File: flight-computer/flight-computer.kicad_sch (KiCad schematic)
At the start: 37 parts, among them J1 Conn_01x06_Pin, J2 Conn_01x06_Pin, J3 Power Connector, J4 Micro_SD_Card, J5 USB_C_Receptacle_USB2.0_16P, J6 Conn_01x02_Pin, Q1 DMN3404L, Q2 DMN3404L, U1 LMR51420X, U2 ESP32-S3-WROOM-1, U3 LSM6DSO32TR, U4 INA2180A1IDGKR

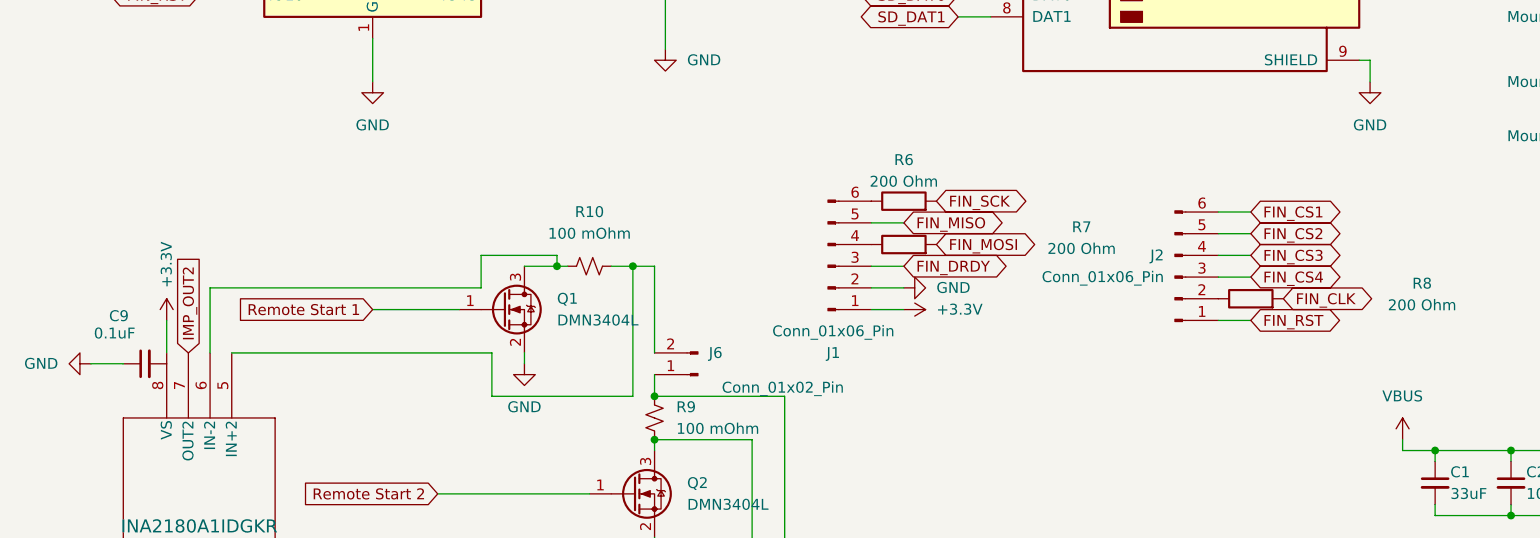
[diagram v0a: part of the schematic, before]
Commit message: finished connecting things
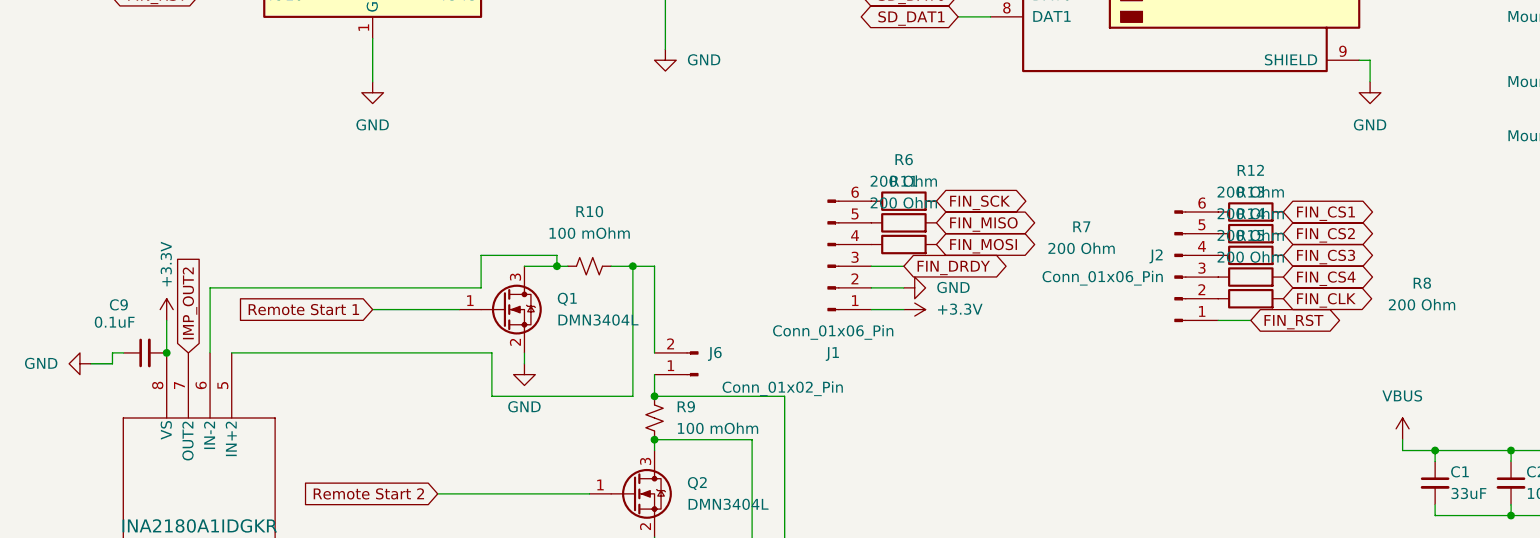
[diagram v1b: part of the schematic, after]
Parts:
- added R11, R12, R13, R14, R15: 200 Ohm, Resistor_SMD:R_0402_1005Metric, symbol Device:R
- J1, J2: footprint Connector_JST:JST_ZH_S6B-ZR-SM4A-TF_1x06-1MP_P1.50mm_Horizontal -> Connector_JST:JST_ZE_S06B-ZESK-2D_1x06_P1.50mm_Horizontal
- R10, R9: footprint Resistor_SMD:R_0402_1005Metric -> Resistor_SMD:R_1206_3216Metric
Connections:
- net +3.3V: now also C9.2
- net FIN_CS1: now also R12.2; no longer J2.6 (Pin_6)
- net FIN_CS2: now also R13.2; no longer J2.5 (Pin_5)
- net FIN_CS3: now also R14.2; no longer J2.4 (Pin_4)
- net FIN_CS4: now also R15.2; no longer J2.3 (Pin_3)
- net FIN_MISO: now also R11.2; no longer J1.5 (Pin_5)
- new net: J1.5 (Pin_5), R11.1
- new net: J2.3 (Pin_3), R15.1
- new net: J2.4 (Pin_4), R14.1
- new net: J2.5 (Pin_5), R13.1
- new net: J2.6 (Pin_6), R12.1
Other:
- moved on the sheet: C9

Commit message: started organizing
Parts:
- J1, J2: footprint Connector_JST:JST_ZE_S06B-ZESK-2D_1x06_P1.50mm_Horizontal -> Connector_JST:JST_ZE_SM06B-ZESS-TB_1x06-1MP_P1.50mm_Horizontal
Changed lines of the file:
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@@
 			)
 		)
-		(property "Footprint" "Connector_JST:JST_ZE_S06B-ZESK-2D_1x06_P1.50mm_Horizontal"
+		(property "Footprint" "Connector_JST:JST_ZE_SM06B-ZESS-TB_1x06-1MP_P1.50mm_Horizontal"
 			(at 163.83 116.84 0)
 			(effects
@@
 			)
 		)
-		(property "Footprint" "Connector_JST:JST_ZE_S06B-ZESK-2D_1x06_P1.50mm_Horizontal"
+		(property "Footprint" "Connector_JST:JST_ZE_SM06B-ZESS-TB_1x06-1MP_P1.50mm_Horizontal"
 			(at 123.19 115.57 0)
 			(effects
